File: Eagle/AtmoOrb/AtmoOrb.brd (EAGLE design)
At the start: 40.6 x 50.8 mm, 10 parts, among them J1 DCJ0202

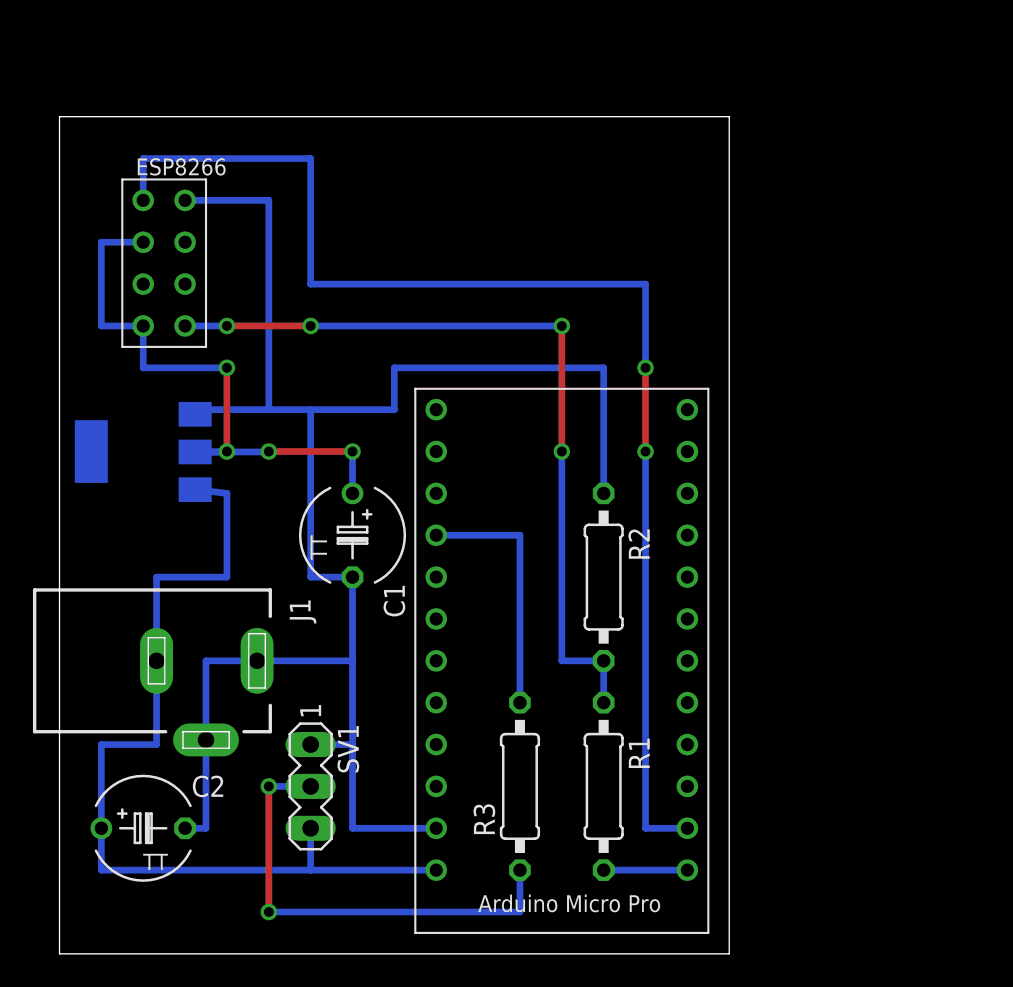
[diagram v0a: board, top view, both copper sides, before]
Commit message: Updated schematic and board layout
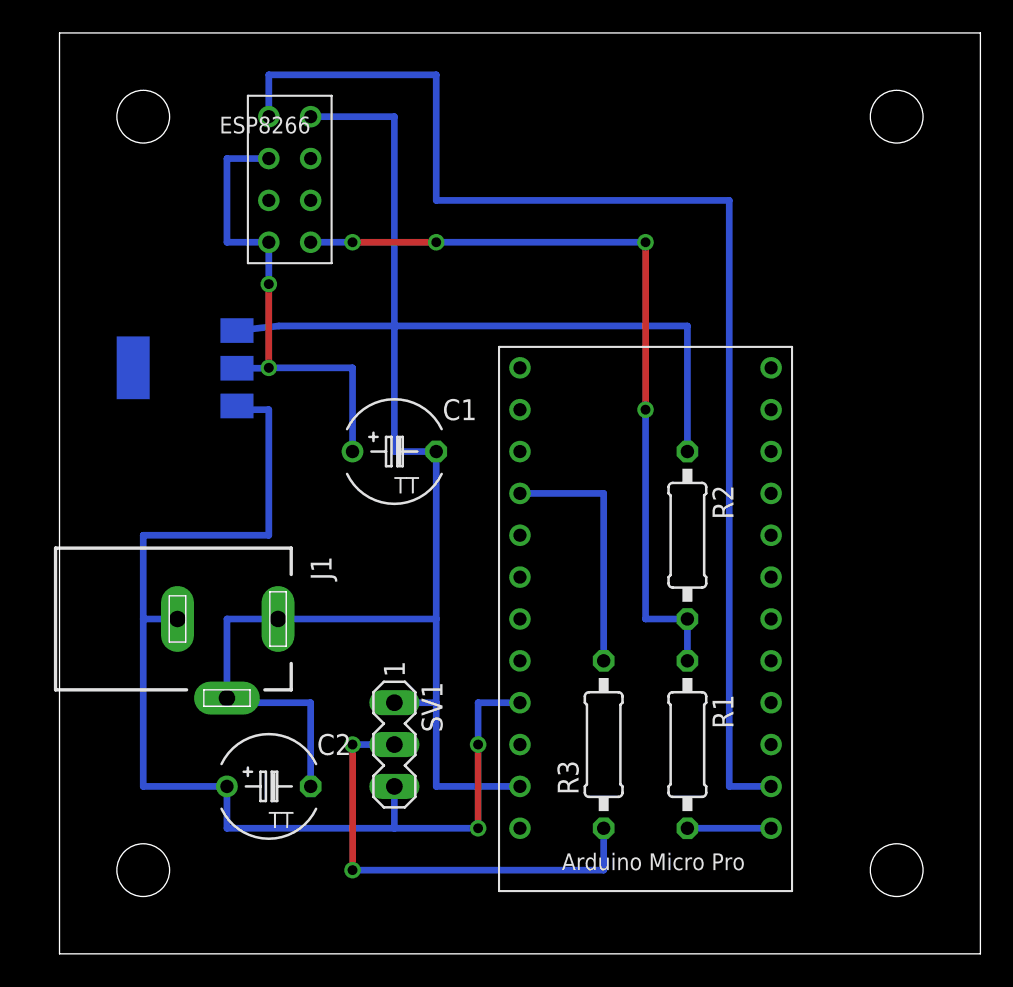
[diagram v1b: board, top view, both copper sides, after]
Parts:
- moved ESP8266 9.16 mm to (12.7, 50.8)
- moved C2 8.03 mm to (12.7, 10.2)
- moved AMS1117 5.68 mm to (7.62, 35.6)
- moved C1 5.68 mm to (20.3, 30.5), turned to 0 degrees
- moved R3 5.68 mm to (33.0, 12.7)
- moved SV1 5.68 mm to (20.3, 12.7)
- moved ARDUINO-MICRO-PRO 5.68 mm to (43.2, 7.62)
- moved R1 5.68 mm to (38.1, 12.7)
- moved R2 5.68 mm to (38.1, 25.4)
- moved J1 2.84 mm to (10.2, 20.3)
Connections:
- net +5V: now also ARDUINO-MICRO-PRO.4; no longer ARDUINO-MICRO-PRO.1
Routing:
- net +5V: track 55.3 -> 70.3 mm, vias 0 -> 2
- net GND: track 108.9 -> 118.8 mm
- net +3V3: track 36.9 -> 29.9 mm, vias 4 -> 2
- net N$3: vias 2 -> 0
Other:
- board size 40.6 x 50.8 mm -> 55.9 x 55.9 mm
